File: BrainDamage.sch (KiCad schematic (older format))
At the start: 52 parts, among them CON1 AVR-ISP-10, IC1 ATMEGA328P-A, J1 TEST_2P, J10 Conn_01x02, J11 Conn_01x04, J12 Conn_01x04, J2 TEST_2P, J3 TEST_2P, J4 TEST_2P, J5 TEST_2P, J6 TEST_2P, J7 15A, J8 Bluetooth, J9 USB_OTG, P8 CONN_01X08, SW1 SW_PUSH, U1 PCA9685-TSSOP, U2 CH340G, U3 AP1117-50, X1 CRYSTAL_SMD, X2 CRYSTAL_SMD

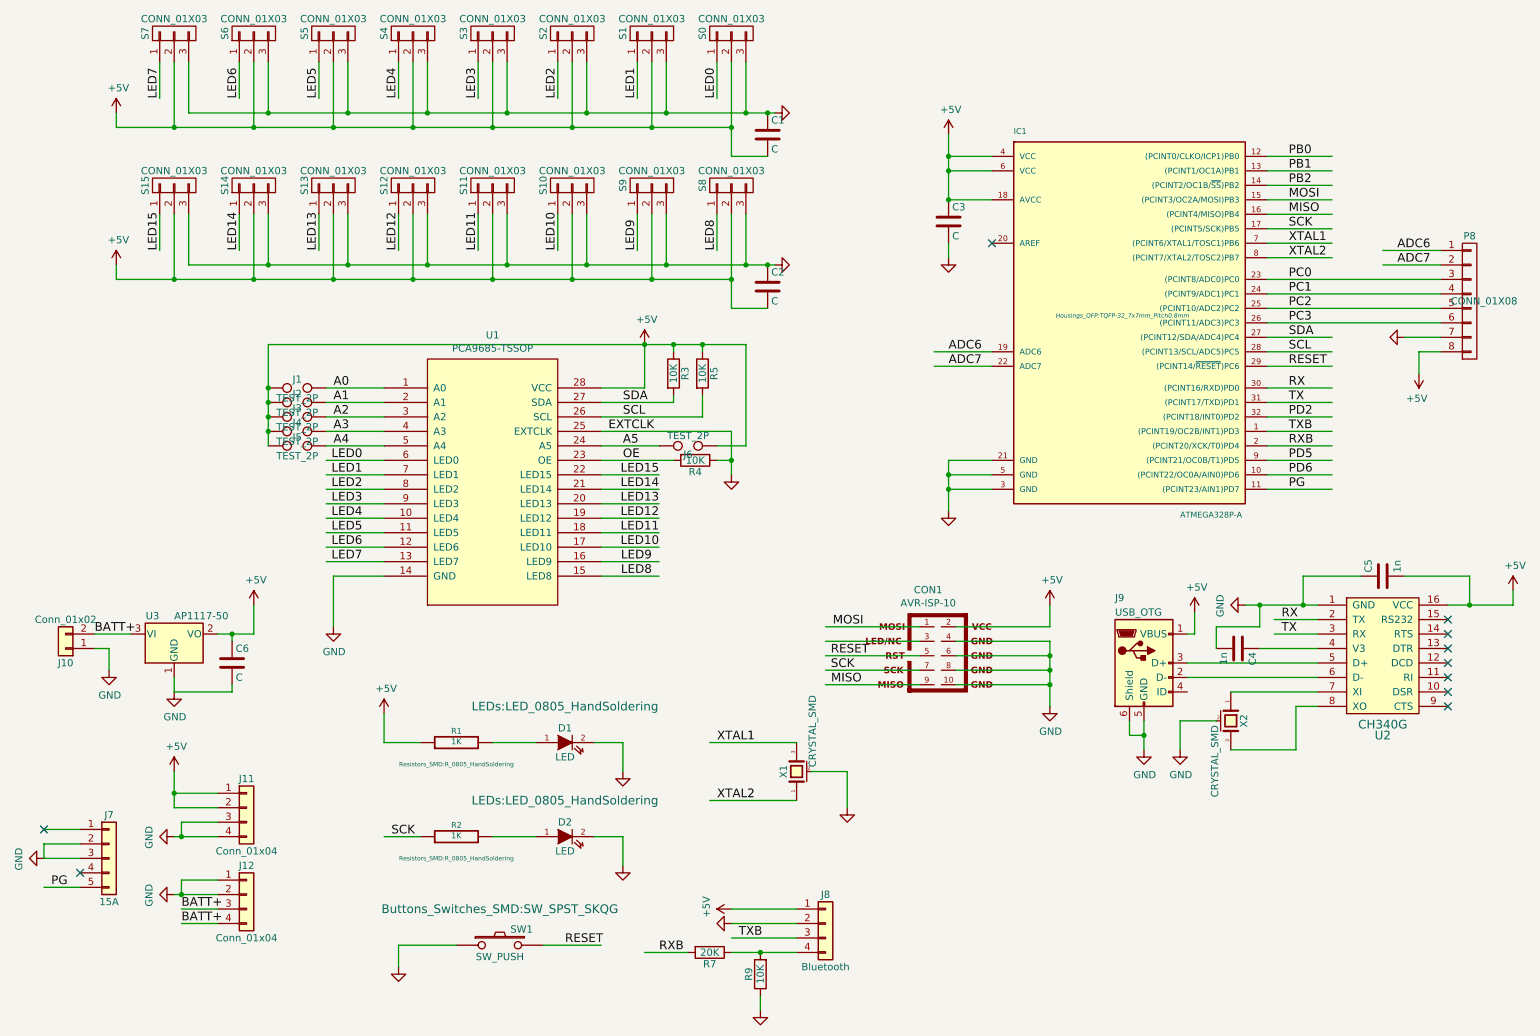
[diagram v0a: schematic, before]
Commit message: Add files via upload
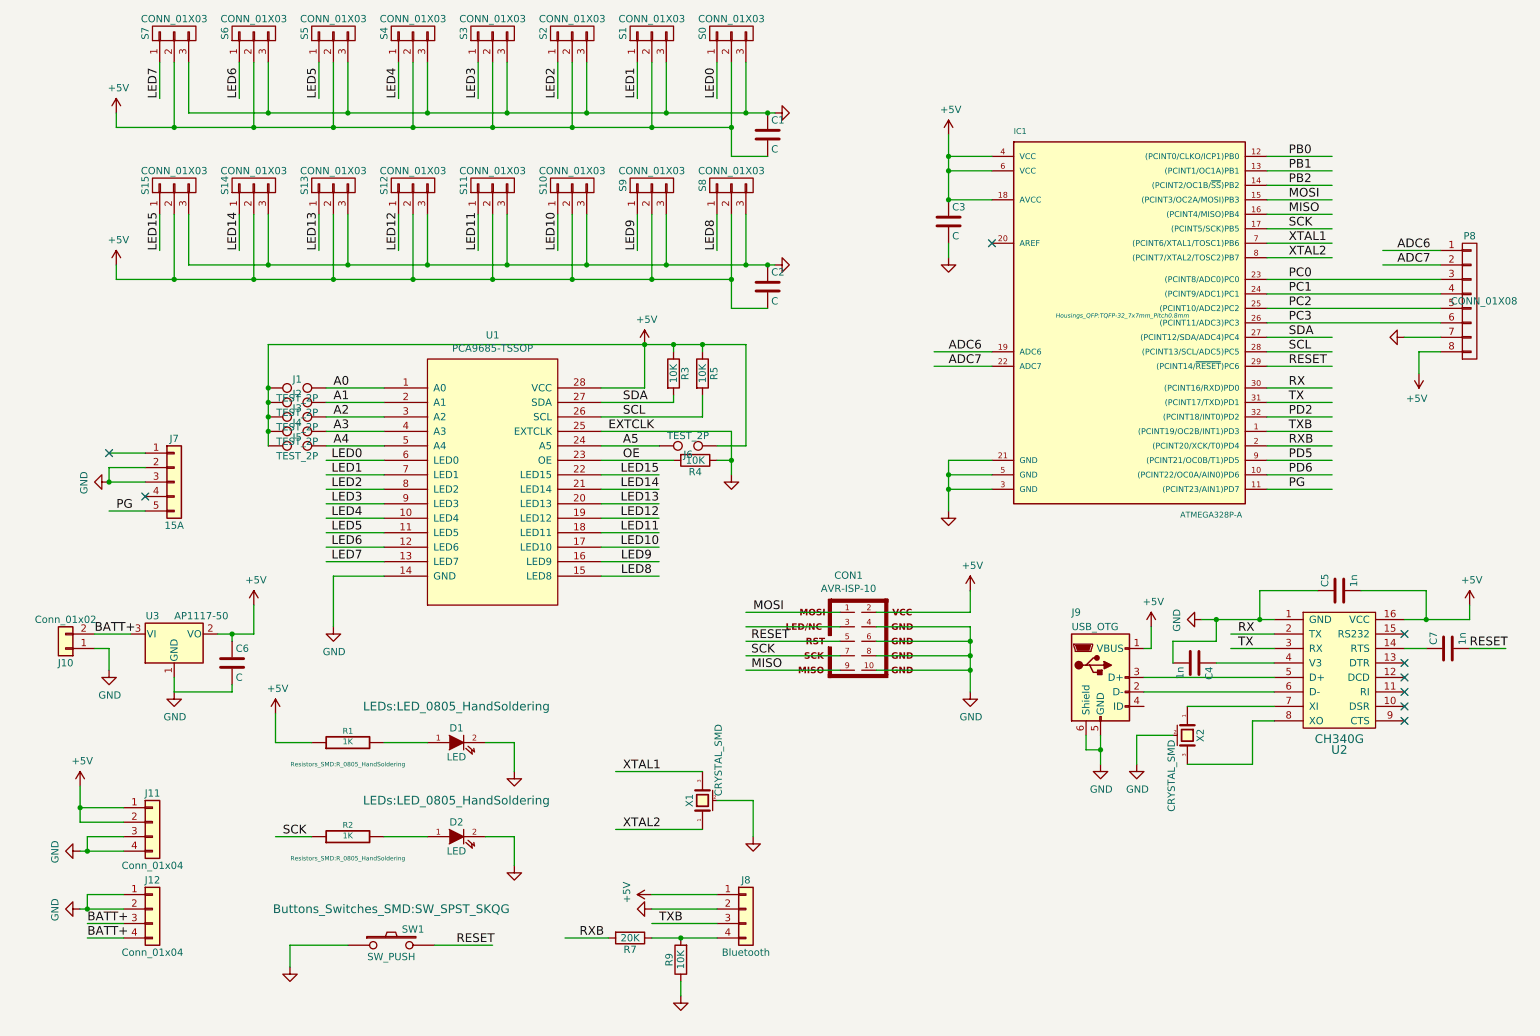
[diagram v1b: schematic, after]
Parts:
- added C7: 1n, Capacitors_SMD:C_0805_HandSoldering, symbol device:C
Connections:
- wire segments 276 -> 278
- no-connect marks 10 -> 9
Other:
- moved on the sheet: C4, C5, CON1, D1, D2, J11, J12, J7, J8, J9, R1, R2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
